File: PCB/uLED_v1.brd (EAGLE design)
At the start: 27.9 x 27.9 mm, 17 parts, among them IC1 ATSAMD21E, J2 455-1750-1-ND, SW1 EG1218, U1 AP2112K-3.3

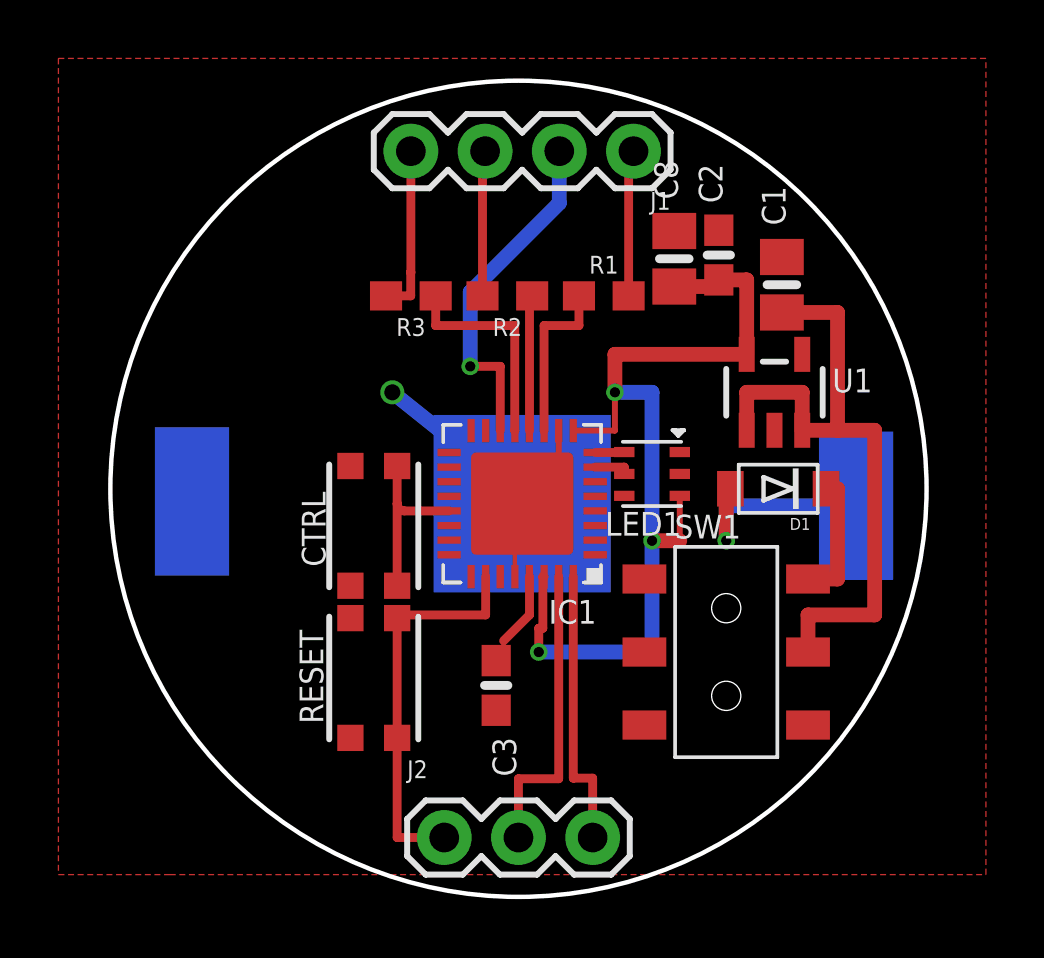
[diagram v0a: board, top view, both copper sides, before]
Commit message: Saturday Morning Commit
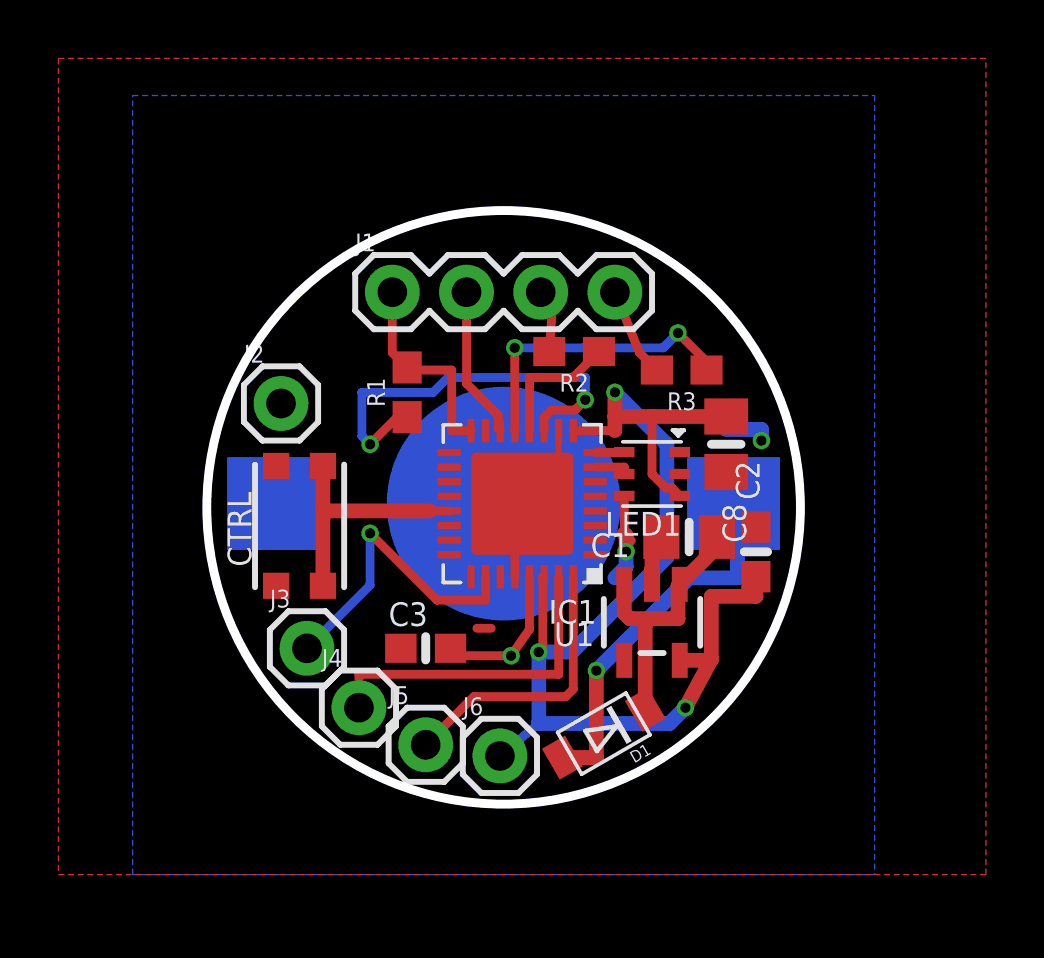
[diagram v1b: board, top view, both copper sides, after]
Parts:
- removed RESET: (no value), microbuilder:BTN_KMR2_4.6X2.8
- removed SW1: EG1218, microbuilder:EG1390
- removed U$3: 20MM_BATTERY, mikes:BATTCON_20MM
- added BT1: (no value), SparkFun-Batteries:BATTCON_12MM
- added J3, J4, J5, J6: (no value), SparkFun-Connectors:1X01
- J2: value 455-1750-1-ND -> (none); device SparkFun-Connectors:1X03 -> SparkFun-Connectors:1X01
- moved J2 15.9 mm to (40.6, 27.6)
- moved D1 10.3 mm to (51.7, 16.3), turned to 210 degrees
- moved C2 10.2 mm to (56.9, 22.5)
- moved R3 9.61 mm to (54.4, 28.7)
- moved J1 9.56 mm to (44.5, 31.4), turned to 0 degrees
- moved C1 9.20 mm to (54.6, 23.0), turned to 180 degrees
- moved U1 8.92 mm to (53.3, 20.1), turned to 180 degrees
- moved R1 7.50 mm to (45.0, 27.9), turned to 90 degrees
- moved C8 6.59 mm to (55.9, 26.2), turned to 270 degrees
- moved R2 2.98 mm to (50.7, 29.3)
- moved C3 2.73 mm to (45.6, 19.2), turned to 180 degrees
- moved CTRL 2.54 mm to (41.3, 23.4)
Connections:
- net N$2 renamed BLUELED
- net N$3 renamed GREENLED
- removed net +1: U$3.1
- removed net N$1: J1.1, R1.2
- removed net SERCOM_1+3.0: IC1.17
- removed net SERCOM_1+3.1: IC1.18
- removed net VOUT: C1.1, SW1.P1, U1.1, U1.3
- new net REDLED: IC1.16, J1.1, R1.2
- net 3.3V: now also J6.1
- net GND: now also BT1.GND, J2.1; no longer RESET.B, RESET.B', U$3.2
- net RESETN: now also J3.1; no longer J2.1, RESET.A, RESET.A'
- net SCDIO: now also J5.1; no longer J2.3
- net SWCLK: now also J4.1; no longer J2.2
- net VBAT: now also BT1.PWR@1; no longer U$3.3
- net VHIGH: now also C1.1, U1.1, U1.3; no longer SW1.O1
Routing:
- net VOUT: track 22.8 -> 0.00 mm
- net 3.3V: track 33.1 -> 42.6 mm
- net REDOUT: track 5.81 -> 14.3 mm, vias 0 -> 2
- net REDLED: track 0.00 -> 7.14 mm
- net ANODE: track 11.9 -> 5.22 mm, vias 1 -> 0
- net BUTTON: track 5.98 -> 12.5 mm
- net VBAT: track 7.56 -> 12.9 mm
- net N$1: track 5.12 -> 0.00 mm
- net VHIGH: track 4.49 -> 9.46 mm
- net RESETN: track 13.6 -> 10.5 mm, vias 0 -> 1
- net BLUEOUT: track 7.32 -> 10.3 mm, vias 0 -> 2
- net GREENLED: track 5.04 -> 2.19 mm
- net BLUELED: track 5.80 -> 3.08 mm
- net VDDCORE: track 3.34 -> 5.05 mm, vias 0 -> 1
- net GND: track 11.5 -> 12.8 mm, vias 1 -> 2
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- added copper zone on layer 16, net GND
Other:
- board size 27.9 x 27.9 mm -> 20.3 x 20.3 mm
